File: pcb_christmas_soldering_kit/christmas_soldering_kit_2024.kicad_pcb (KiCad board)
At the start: 2 copper layers, 79.8 x 99.3 mm, 17 parts, among them P1 Conn_01x08_Pin, P2 Conn_01x08_Pin, SW1 Button, U1 ESP32-C3

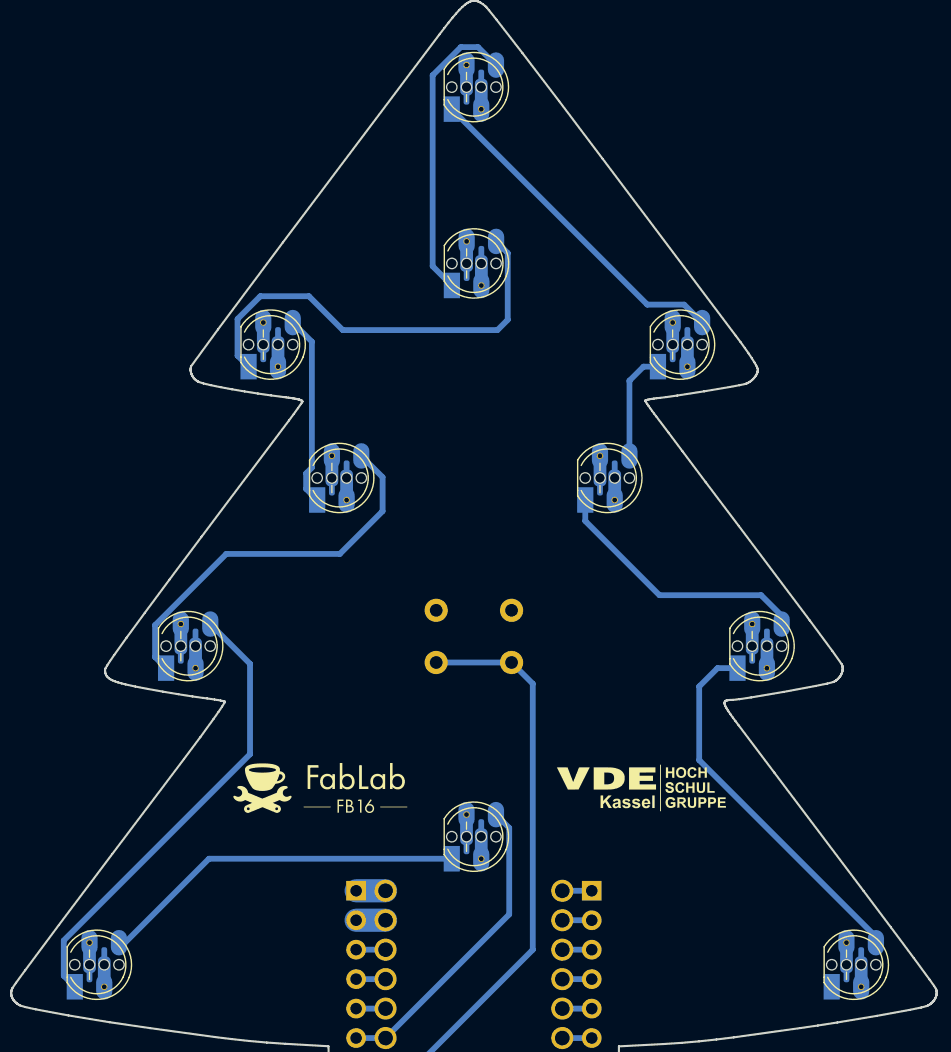
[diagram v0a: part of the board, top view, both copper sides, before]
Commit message: prototype 2 (ordered)
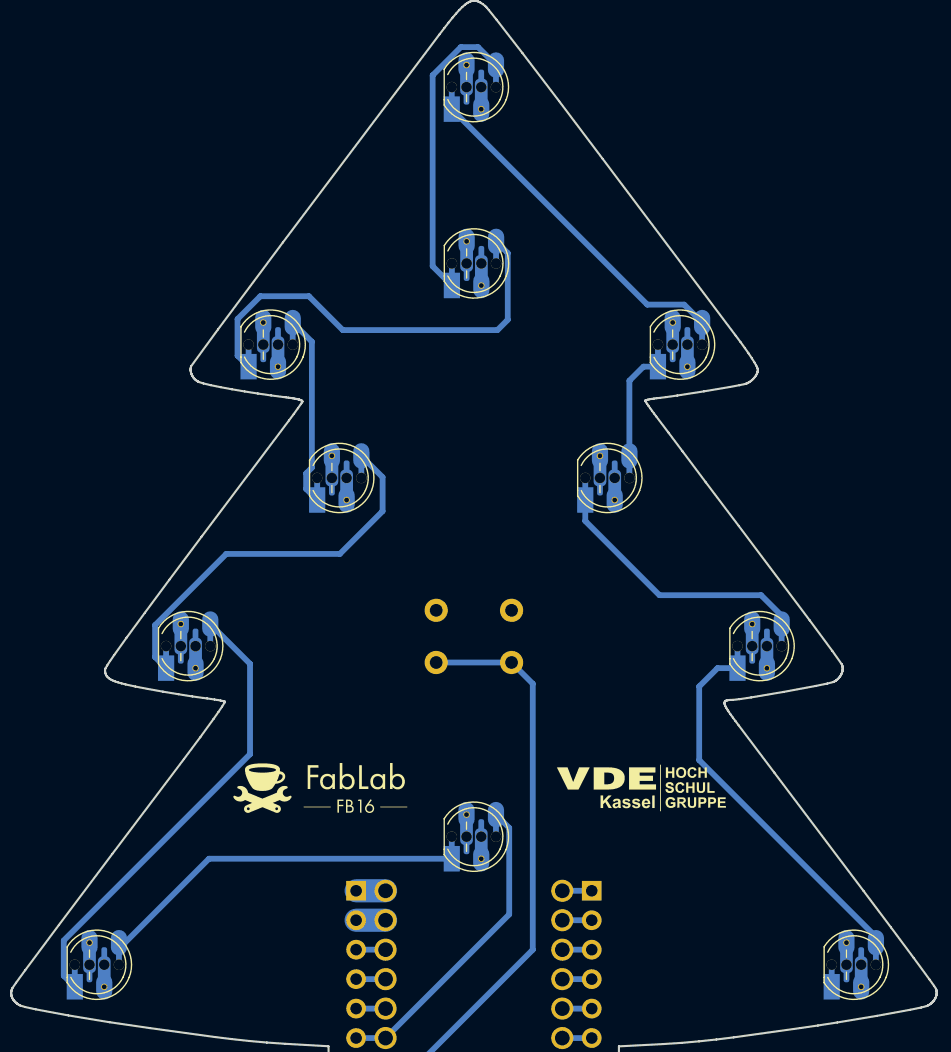
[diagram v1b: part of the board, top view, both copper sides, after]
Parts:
- D1, D10, D11, D2, D3, D4, D5, D6, D7, D8, D9: footprint Library:LED_D5.0mm-4_RGB_easy -> Library:LED_D5.0mm-4_RGB_easy_2

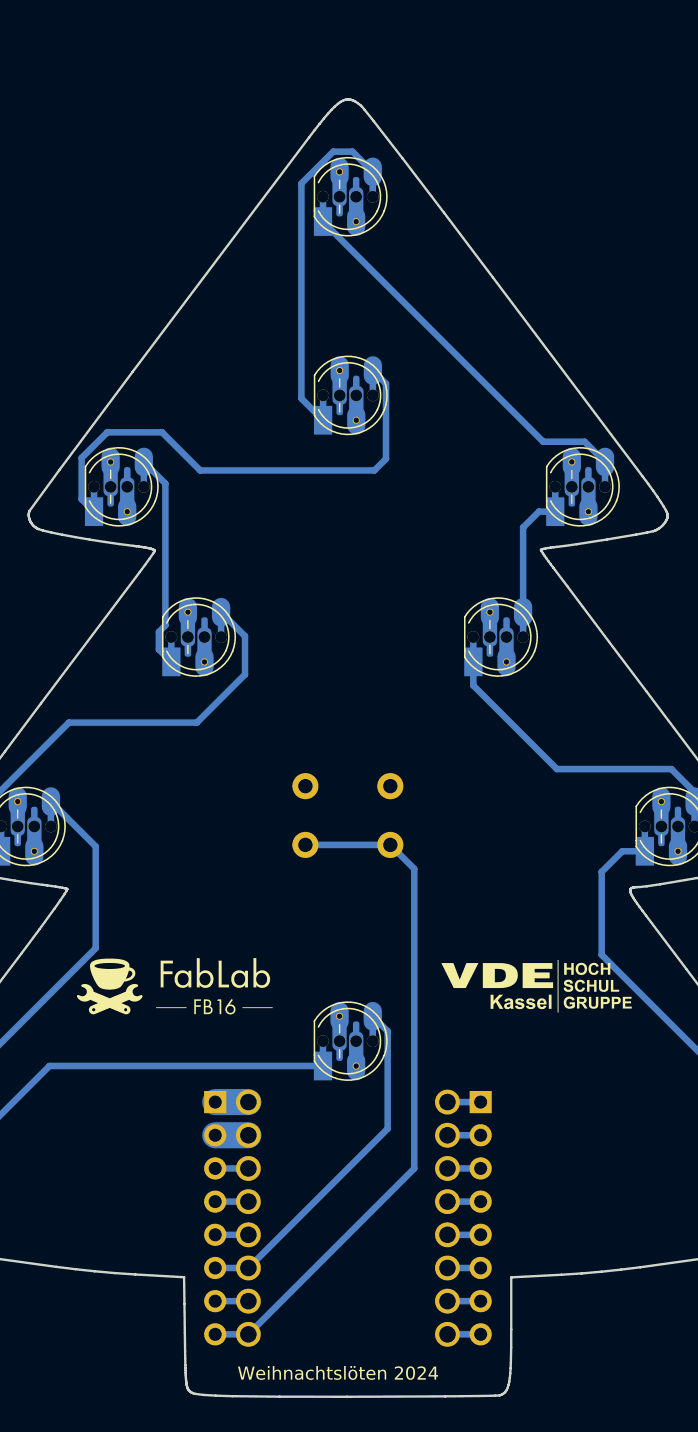
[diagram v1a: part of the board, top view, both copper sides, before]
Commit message: final version, rev. 1.0: ordered
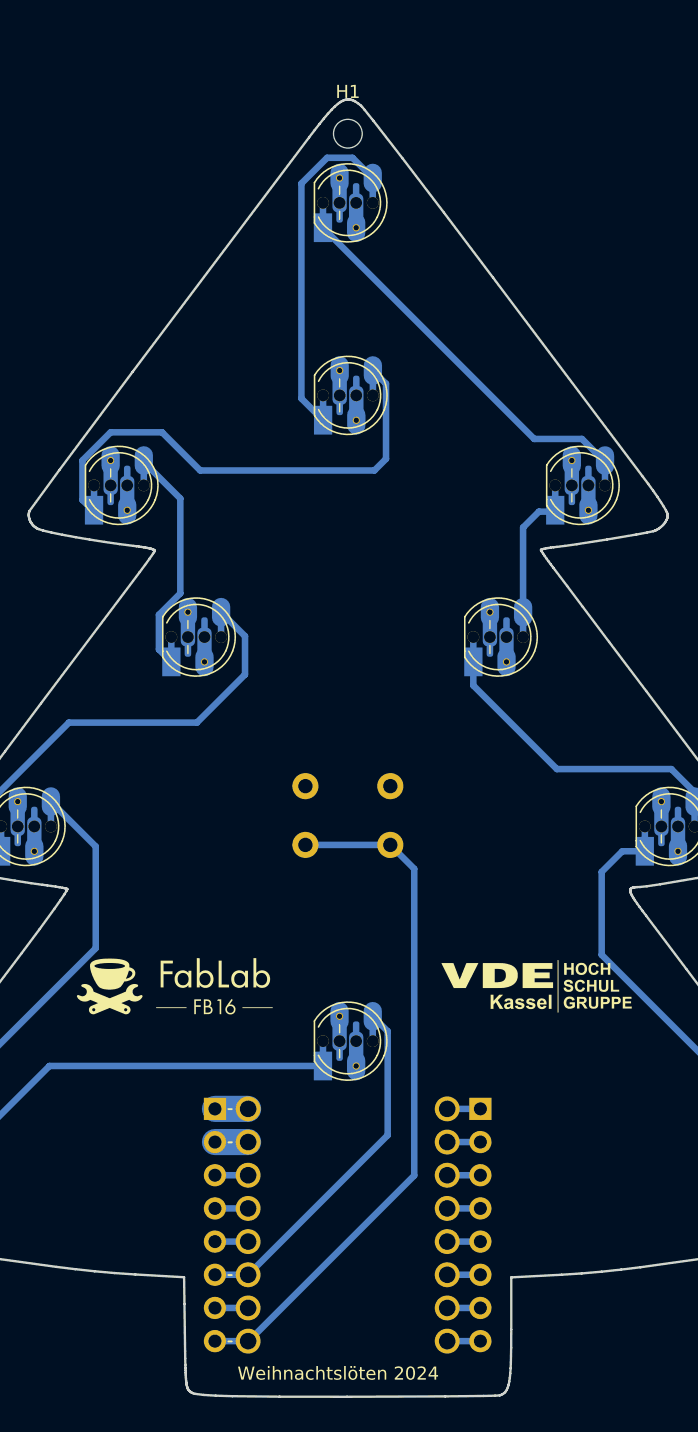
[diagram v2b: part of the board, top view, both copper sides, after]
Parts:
- added H1: MountingHole, MountingHole:MountingHole_2.2mm_M2, F.Cu at (150.5, 45.5)
- moved P1 0.52 mm to (140.3, 120.1)
- moved P2 0.52 mm to (160.6, 120.1)
- moved U1 0.52 mm to (150.5, 130.0)
- moved D7 0.47 mm to (148.6, 50.8)
- moved D5 0.11 mm to (131.1, 72.4)
- moved D8 0.11 mm to (166.4, 72.4)
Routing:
- net Net-(D4-DO): track 16.6 -> 17.5 mm
- net GPIO2: track 26.7 -> 27.2 mm
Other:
- board text added: "Rev. 1.0"
- board text removed: "Prototyp 2"
